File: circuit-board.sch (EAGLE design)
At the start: 42 parts, among them Q1 BC547B, U1 MAX3232, U2 ATMEGA328P_TQFP, U3 ADUM1201BRZ, U4 UA78M05CDCY, Y1 16MHz

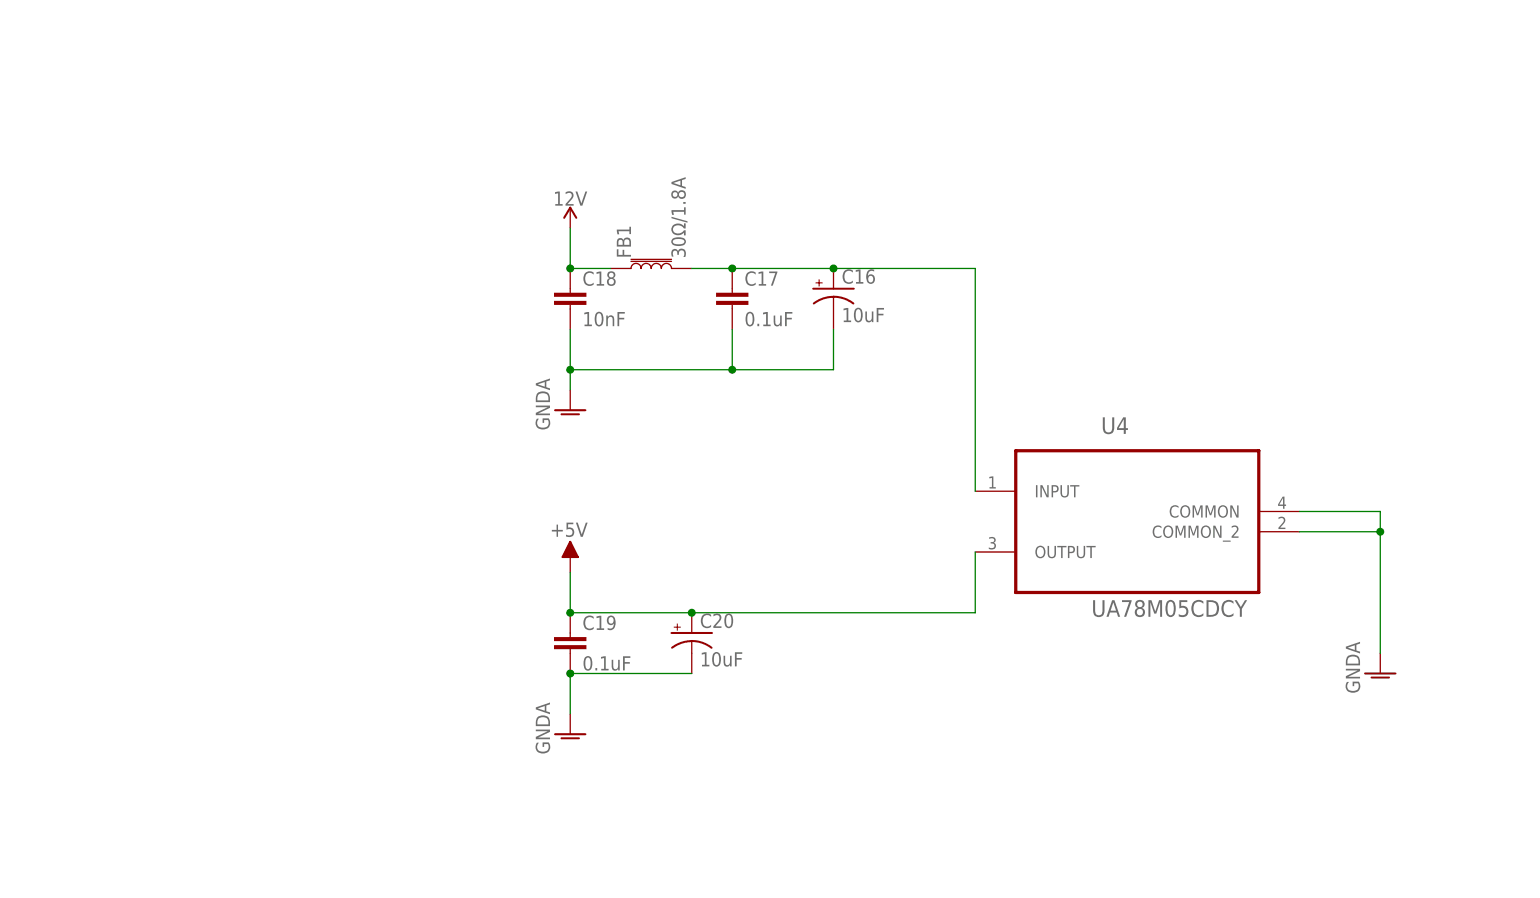
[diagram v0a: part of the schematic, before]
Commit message: Board is final, sending to fab shop
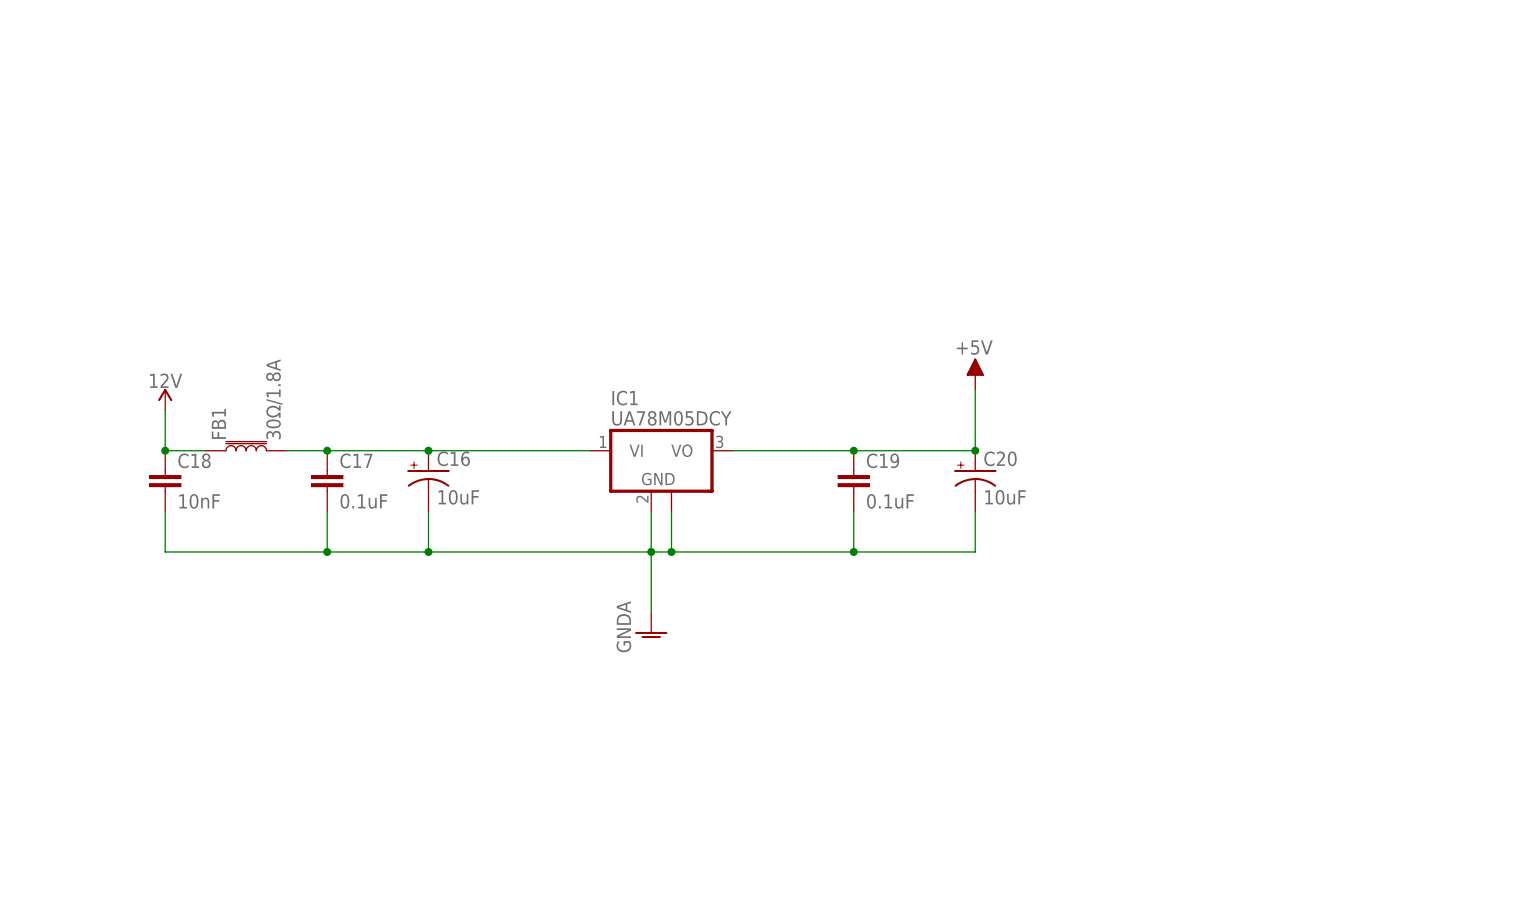
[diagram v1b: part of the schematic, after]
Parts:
- removed U4: UA78M05CDCY, Texas Instruments_By_element14_Batch_1:UA78M05CDCY
- added IC1: UA78M05DCY, linear:UA78M05DCY
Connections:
- net +5V: now also IC1.VO; no longer U4.OUTPUT
- net GNDA: now also IC1.GND, IC1.GND@1; no longer U4.COMMON, U4.COMMON_2
- net N$1: now also IC1.VI; no longer U4.INPUT
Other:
- moved on the sheet: C16, C17, C18, C19, C20, FB1
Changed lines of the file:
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@@
 <part name="C17" library="SparkFun-Capacitors" deviceset="0.1UF" device="-0603-25V-5%" value="0.1uF"/>
 <part name="C18" library="SparkFun-Capacitors" library_urn="urn:adsk.eagle:library:510" deviceset="10NF" device="-0603-50V-10%" package3d_urn="urn:adsk.eagle:package:37414/1" value="10nF"/>
-<part name="U4" library="Texas Instruments_By_element14_Batch_1" deviceset="UA78M05CDCY" device=""/>
-<part name="GND22" library="supply1" deviceset="GNDA" device=""/>
 <part name="GND5" library="supply1" deviceset="GNDA" device=""/>
 <part name="SUPPLY3" library="SparkFun-PowerSymbols" deviceset="12V" device=""/>
@@
 <part name="C19" library="SparkFun-Capacitors" deviceset="0.1UF" device="-0603-25V-5%" value="0.1uF"/>
 <part name="C20" library="adafruit" library_urn="urn:adsk.eagle:library:420" deviceset="CPOL-US" device="E2.5-5" value="10uF"/>
-<part name="GND23" library="supply1" deviceset="GNDA" device=""/>
+<part name="IC1" library="linear" library_urn="urn:adsk.eagle:library:262" deviceset="UA78M*" device="DCY" package3d_urn="urn:adsk.eagle:package:16418/2" technology="05"/>
 </parts>
 <sheets>
@@
 <instance part="GND11" gate="1" x="-177.8" y="172.72" rot="R90"/>
 <instance part="R6" gate="G$1" x="-78.74" y="271.78"/>
-<instance part="FB1" gate="G$1" x="78.74" y="243.84" rot="R90"/>
-<instance part="C16" gate="G$1" x="101.6" y="241.3"/>
-<instance part="C17" gate="G$1" x="88.9" y="238.76"/>
-<instance part="C18" gate="G$1" x="68.58" y="238.76"/>
-<instance part="U4" gate="A" x="139.7" y="215.9"/>
-<instance part="GND22" gate="1" x="170.18" y="193.04"/>
+<instance part="FB1" gate="G$1" x="27.94" y="220.98" rot="R90"/>
+<instance part="C16" gate="G$1" x="50.8" y="218.44"/>
+<instance part="C17" gate="G$1" x="38.1" y="215.9"/>
+<instance part="C18" gate="G$1" x="17.78" y="215.9"/>
 <instance part="GND5" gate="1" x="-271.78" y="243.84" rot="R270"/>
-<instance part="SUPPLY3" gate="G$1" x="68.58" y="248.92"/>
-<instance part="GND8" gate="1" x="68.58" y="226.06"/>
-<instance part="V3" gate="1" x="68.58" y="208.28"/>
-<instance part="C19" gate="G$1" x="68.58" y="195.58"/>
-<instance part="C20" gate="G$1" x="83.82" y="198.12"/>
-<instance part="GND23" gate="1" x="68.58" y="185.42"/>
+<instance part="SUPPLY3" gate="G$1" x="17.78" y="226.06"/>
+<instance part="GND8" gate="1" x="78.74" y="198.12"/>
+<instance part="V3" gate="1" x="119.38" y="231.14"/>
+<instance part="C19" gate="G$1" x="104.14" y="215.9"/>
+<instance part="C20" gate="G$1" x="119.38" y="218.44"/>
+<instance part="IC1" gate="G$1" x="78.74" y="220.98"/>
 </instances>
 <busses>
@@
 <segment>
 <pinref part="C18" gate="G$1" pin="2"/>
+<wire x1="17.78" y1="213.36" x2="17.78" y2="208.28" width="0.1524" layer="91"/>
+<pinref part="C16" gate="G$1" pin="-"/>
+<wire x1="50.8" y1="213.36" x2="50.8" y2="208.28" width="0.1524" layer="91"/>
+<wire x1="50.8" y1="208.28" x2="38.1" y2="208.28" width="0.1524" layer="91"/>
+<pinref part="C17" gate="G$1" pin="2"/>
+<wire x1="38.1" y1="208.28" x2="17.78" y2="208.28" width="0.1524" layer="91"/>
+<wire x1="38.1" y1="213.36" x2="38.1" y2="208.28" width="0.1524" layer="91"/>
+<junction x="38.1" y="208.28"/>
+<pinref part="C19" gate="G$1" pin="2"/>
+<wire x1="104.14" y1="213.36" x2="104.14" y2="208.28" width="0.1524" layer="91"/>
+<wire x1="50.8" y1="208.28" x2="78.74" y2="208.28" width="0.1524" layer="91"/>
+<junction x="50.8" y="208.28"/>
+<pinref part="IC1" gate="G$1" pin="GND"/>
+<wire x1="78.74" y1="208.28" x2="81.28" y2="208.28" width="0.1524" layer="91"/>
+<wire x1="81.28" y1="208.28" x2="104.14" y2="208.28" width="0.1524" layer="91"/>
+<wire x1="78.74" y1="213.36" x2="78.74" y2="208.28" width="0.1524" layer="91"/>
+<junction x="78.74" y="208.28"/>
+<pinref part="IC1" gate="G$1" pin="GND@1"/>
+<wire x1="81.28" y1="213.36" x2="81.28" y2="208.28" width="0.1524" layer="91"/>
+<junction x="81.28" y="208.28"/>
 <pinref part="GND8" gate="1" pin="GNDA"/>
-<wire x1="68.58" y1="236.22" x2="68.58" y2="231.14" width="0.1524" layer="91"/>
-<pinref part="C16" gate="G$1" pin="-"/>
-<wire x1="68.58" y1="231.14" x2="68.58" y2="228.6" width="0.1524" layer="91"/>
-<wire x1="101.6" y1="236.22" x2="101.6" y2="231.14" width="0.1524" layer="91"/>
-<wire x1="101.6" y1="231.14" x2="88.9" y2="231.14" width="0.1524" layer="91"/>
-<junction x="68.58" y="231.14"/>
-<pinref part="C17" gate="G$1" pin="2"/>
-<wire x1="88.9" y1="231.14" x2="68.58" y2="231.14" width="0.1524" layer="91"/>
-<wire x1="88.9" y1="236.22" x2="88.9" y2="231.14" width="0.1524" layer="91"/>
-<junction x="88.9" y="231.14"/>
-</segment>
-<segment>
-<pinref part="C19" gate="G$1" pin="2"/>
-<pinref part="GND23" gate="1" pin="GNDA"/>
-<wire x1="68.58" y1="193.04" x2="68.58" y2="187.96" width="0.1524" layer="91"/>
+<wire x1="78.74" y1="208.28" x2="78.74" y2="200.66" width="0.1524" layer="91"/>
 <pinref part="C20" gate="G$1" pin="-"/>
-<wire x1="68.58" y1="193.04" x2="83.82" y2="193.04" width="0.1524" layer="91"/>
-<junction x="68.58" y="193.04"/>
-</segment>
-<segment>
-<pinref part="U4" gate="A" pin="COMMON"/>
-<wire x1="160.02" y1="213.36" x2="170.18" y2="213.36" width="0.1524" layer="91"/>
-<pinref part="GND22" gate="1" pin="GNDA"/>
-<wire x1="170.18" y1="213.36" x2="170.18" y2="210.82" width="0.1524" layer="91"/>
-<pinref part="U4" gate="A" pin="COMMON_2"/>
-<wire x1="170.18" y1="210.82" x2="170.18" y2="195.58" width="0.1524" layer="91"/>
-<wire x1="160.02" y1="210.82" x2="170.18" y2="210.82" width="0.1524" layer="91"/>
-<junction x="170.18" y="210.82"/>
+<wire x1="119.38" y1="213.36" x2="119.38" y2="208.28" width="0.1524" layer="91"/>
+<wire x1="119.38" y1="208.28" x2="104.14" y2="208.28" width="0.1524" layer="91"/>
+<junction x="104.14" y="208.28"/>
 </segment>
 </net>
@@
 <pinref part="SUPPLY3" gate="G$1" pin="12V"/>
 <pinref part="C18" gate="G$1" pin="1"/>
-<wire x1="68.58" y1="248.92" x2="68.58" y2="243.84" width="0.1524" layer="91"/>
+<wire x1="17.78" y1="226.06" x2="17.78" y2="220.98" width="0.1524" layer="91"/>
 <pinref part="FB1" gate="G$1" pin="1"/>
-<wire x1="68.58" y1="243.84" x2="73.66" y2="243.84" width="0.1524" layer="91"/>
-<junction x="68.58" y="243.84"/>
+<wire x1="17.78" y1="220.98" x2="22.86" y2="220.98" width="0.1524" layer="91"/>
+<junction x="17.78" y="220.98"/>
 </segment>
 </net>
@@
 </segment>
 <segment>
+<pinref part="C19" gate="G$1" pin="1"/>
+<pinref part="C20" gate="G$1" pin="+"/>
+<wire x1="104.14" y1="220.98" x2="119.38" y2="220.98" width="0.1524" layer="91"/>
 <pinref part="V3" gate="1" pin="+5V"/>
-<pinref part="C19" gate="G$1" pin="1"/>
-<wire x1="68.58" y1="205.74" x2="68.58" y2="200.66" width="0.1524" layer="91"/>
-<pinref part="C20" gate="G$1" pin="+"/>
-<wire x1="68.58" y1="200.66" x2="83.82" y2="200.66" width="0.1524" layer="91"/>
-<junction x="68.58" y="200.66"/>
-<pinref part="U4" gate="A" pin="OUTPUT"/>
-<wire x1="119.38" y1="208.28" x2="119.38" y2="200.66" width="0.1524" layer="91"/>
-<wire x1="119.38" y1="200.66" x2="83.82" y2="200.66" width="0.1524" layer="91"/>
-<junction x="83.82" y="200.66"/>
+<wire x1="119.38" y1="228.6" x2="119.38" y2="220.98" width="0.1524" layer="91"/>
+<junction x="119.38" y="220.98"/>
+<pinref part="IC1" gate="G$1" pin="VO"/>
+<wire x1="104.14" y1="220.98" x2="88.9" y2="220.98" width="0.1524" layer="91"/>
+<junction x="104.14" y="220.98"/>
 </segment>
 </net>
@@
 <pinref part="FB1" gate="G$1" pin="2"/>
 <pinref part="C17" gate="G$1" pin="1"/>
-<wire x1="83.82" y1="243.84" x2="88.9" y2="243.84" width="0.1524" layer="91"/>
+<wire x1="33.02" y1="220.98" x2="38.1" y2="220.98" width="0.1524" layer="91"/>
 <pinref part="C16" gate="G$1" pin="+"/>
-<wire x1="88.9" y1="243.84" x2="101.6" y2="243.84" width="0.1524" layer="91"/>
-<junction x="88.9" y="243.84"/>
-<wire x1="101.6" y1="243.84" x2="119.38" y2="243.84" width="0.1524" layer="91"/>
-<junction x="101.6" y="243.84"/>
-<pinref part="U4" gate="A" pin="INPUT"/>
-<wire x1="119.38" y1="243.84" x2="119.38" y2="215.9" width="0.1524" layer="91"/>
-</segment>
-</net>
+<wire x1="38.1" y1="220.98" x2="50.8" y2="220.98" width="0.1524" layer="91"/>
+<junction x="38.1" y="220.98"/>
+<wire x1="50.8" y1="220.98" x2="71.12" y2="220.98" width="0.1524" layer="91"/>
+<junction x="50.8" y="220.98"/>
+<pinref part="IC1" gate="G$1" pin="VI"/>
+</segment>
+</net>
